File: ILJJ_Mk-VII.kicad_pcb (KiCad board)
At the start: 2 copper layers, 48.3 x 99.1 mm, 27 parts, among them J1 Conn_02x12, U1 74LS00, U10 74LS00, U11 74LS00, U2 74LS00, U3 74LS00, U4 74LS00, U5 74LS00, U6 74LS00, U7 74LS00, U8 74LS00, U9 74LS00

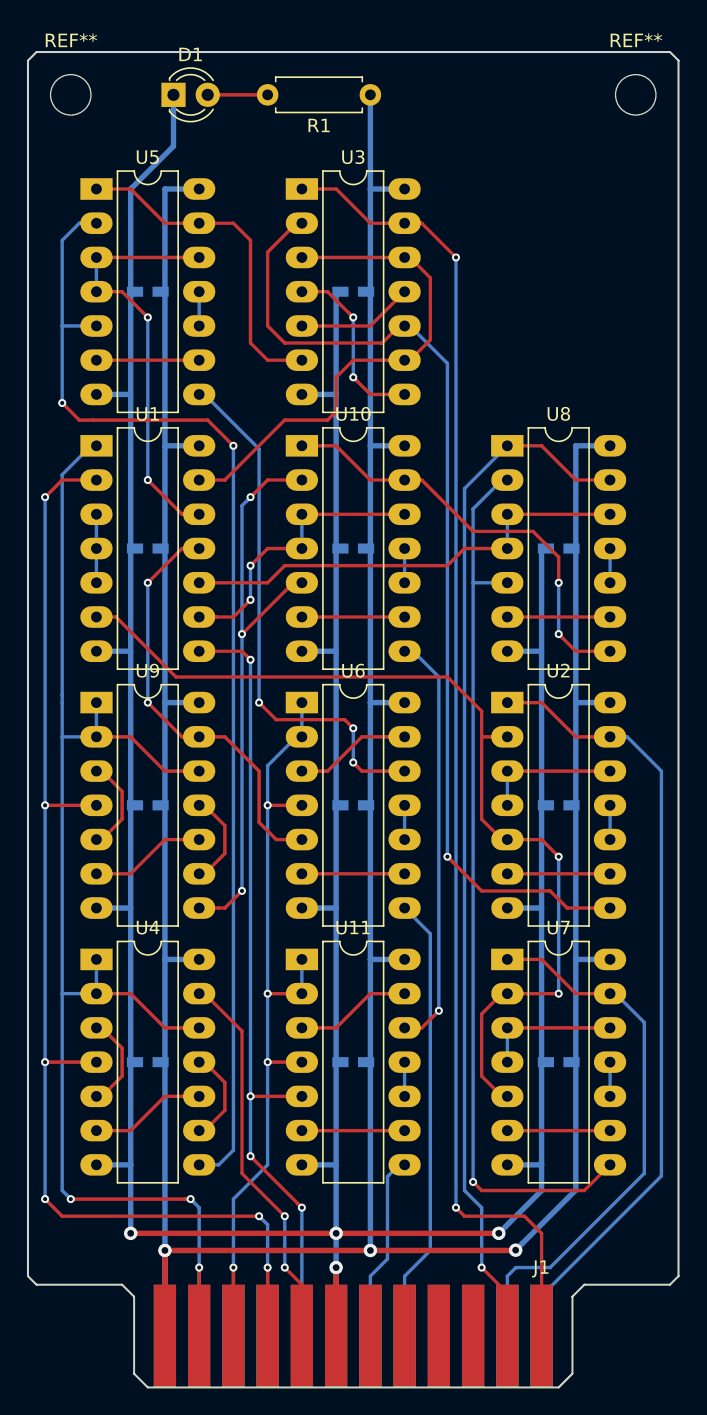
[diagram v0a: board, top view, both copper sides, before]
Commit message: [add] some logos
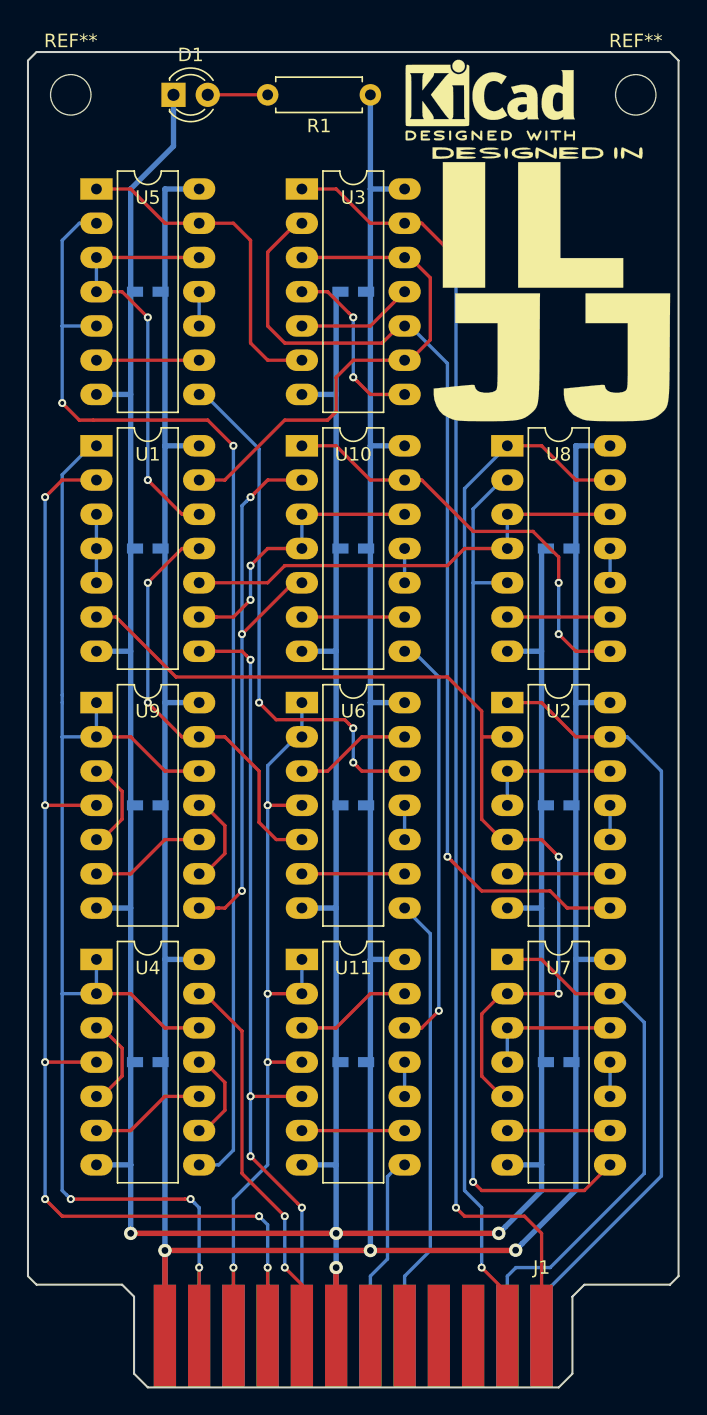
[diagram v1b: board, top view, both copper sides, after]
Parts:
- added G***: LOGO, fplib:designed-in-ILJJ, F.Cu at (140.3, 67.9)
- added REF***: KiCad-Logo2_6mm_SilkScreen, Symbols:KiCad-Logo2_6mm_SilkScreen, F.Cu at (135.9, 54.4)
